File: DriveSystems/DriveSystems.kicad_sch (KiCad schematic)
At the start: 31 parts, among them J1 Raspberry_Pi_4, J2 RJ45, M1 Motor_Servo, M2 Motor_Servo, SW1 SW_Rotary_1x2_MP, U1 RoboClaw Motor Controller, U2 5304 Gear Motor, U3 5VDC 5A UBC-C PSU, U4 24V 5V10A DCDC Stepdown, U5 RoboClaw VClamp, U6 Pwr Res

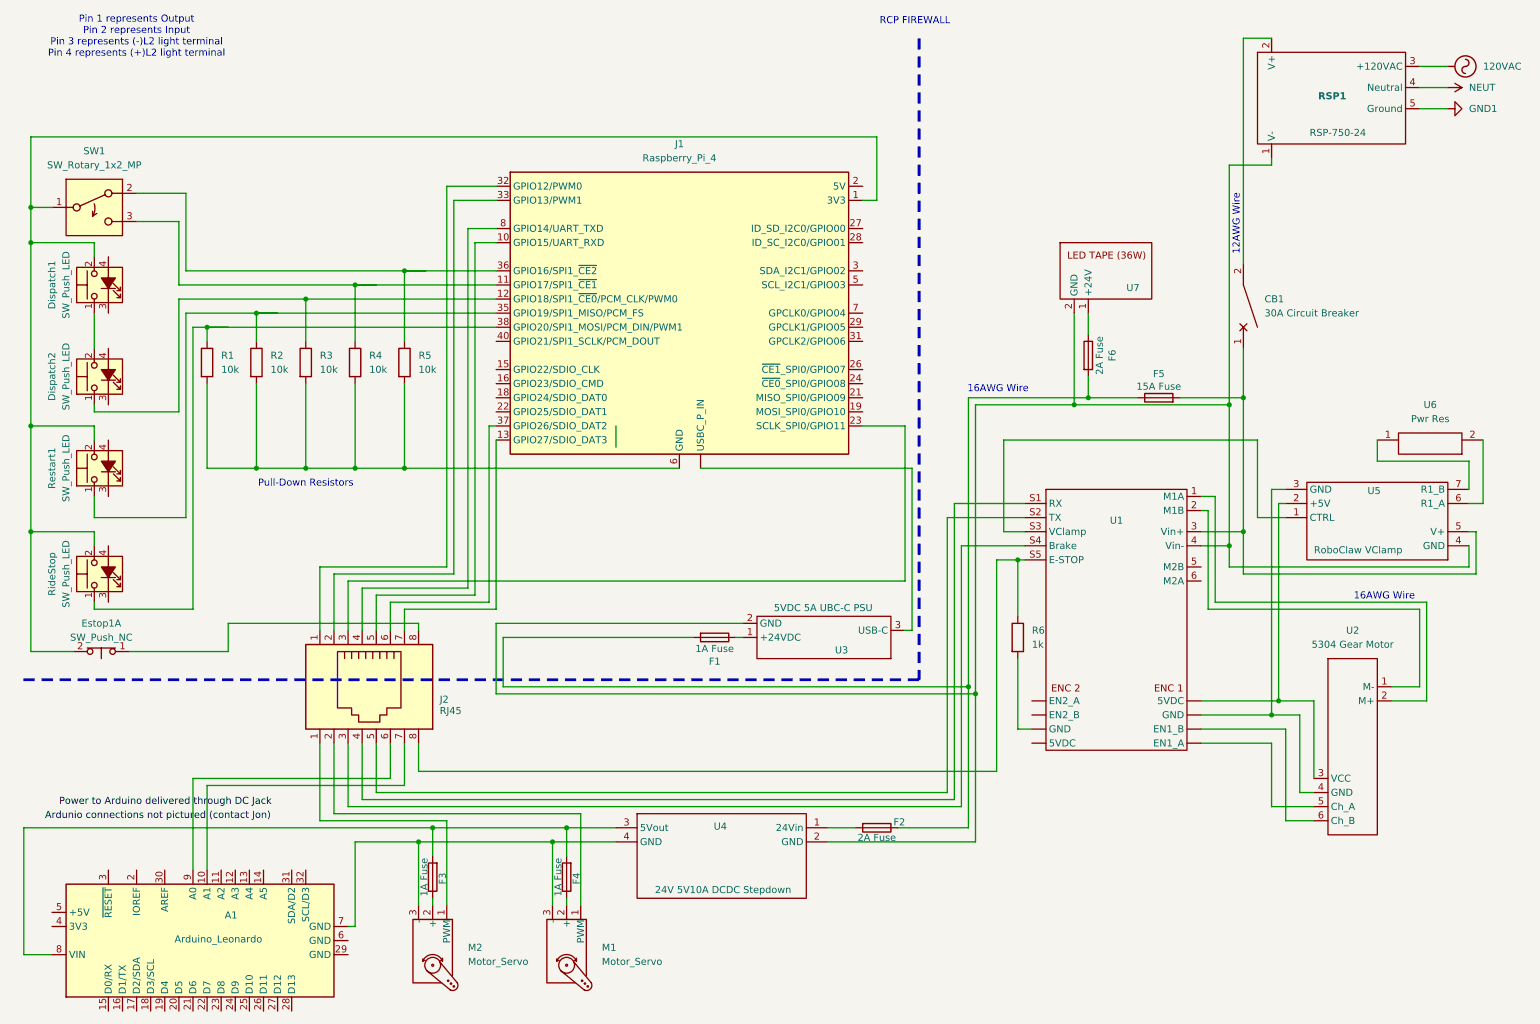
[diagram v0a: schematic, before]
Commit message: Final Cleanup
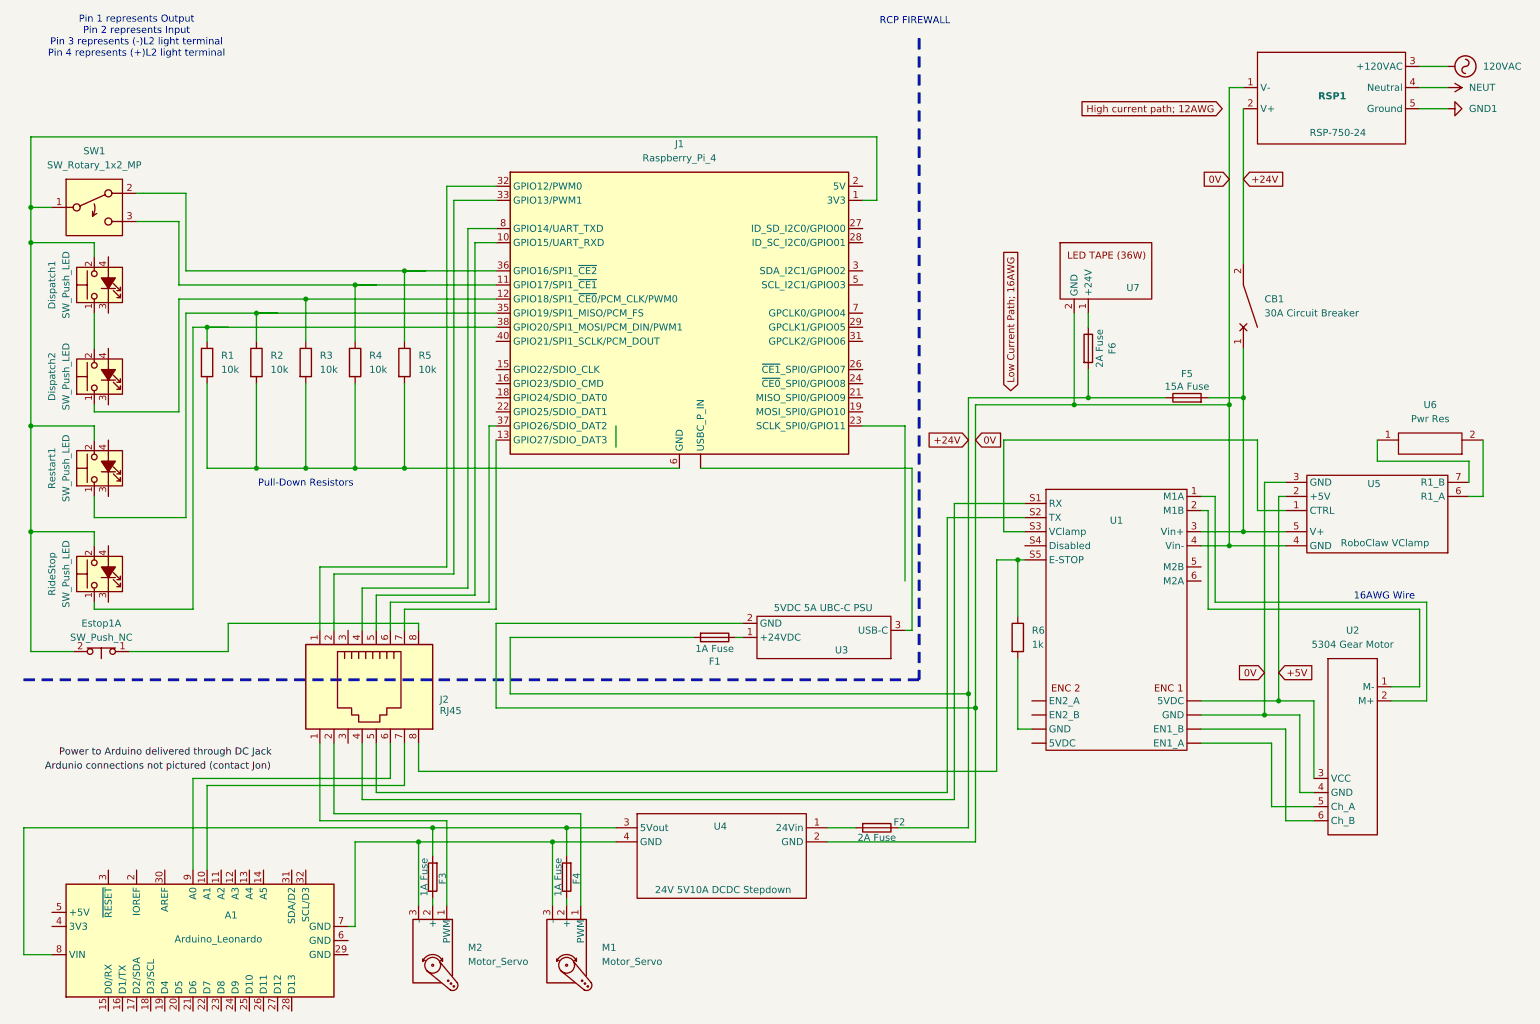
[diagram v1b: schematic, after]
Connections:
- net at J1.23 (SCLK_SPI0/GPIO11): no longer J2.3
- net 0V: now reaches U1. (EN1_A)
- net 0V: now also U1.4 (Vin-), U2.4 (GND), U3.2 (GND), U4.2 (GND), U5.3 (GND), U5.4 (GND), U7.2 (GND)
- net +5V: now reaches U1. (EN1_A), U2.3 (VCC), U5.2 (+5V)
- net at U1.S4 (Disabled): no longer J2.3
- net +24V: now reaches F1.2, F2.1, F5.1, F6.2
- net +24V: now also CB1.2
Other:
- note removed: "12AWG Wire"
- moved on the sheet: F5, F6, U5

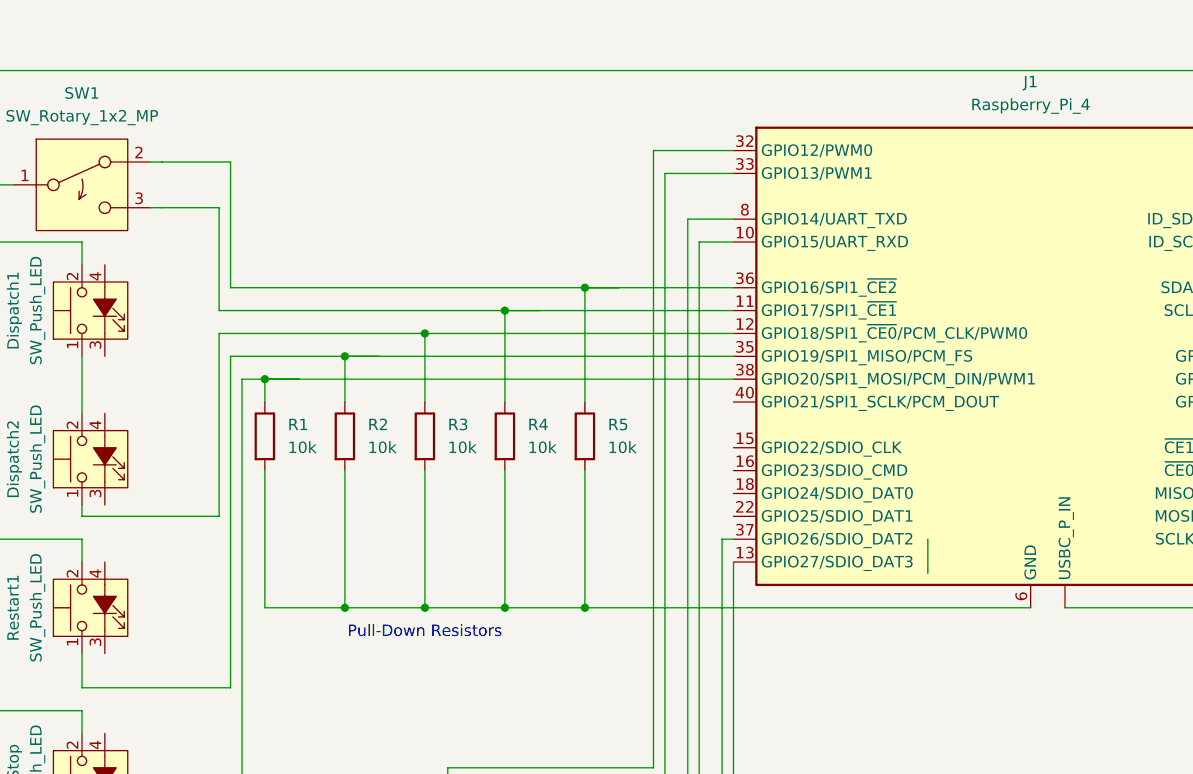
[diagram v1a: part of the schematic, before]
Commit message: NO Switch
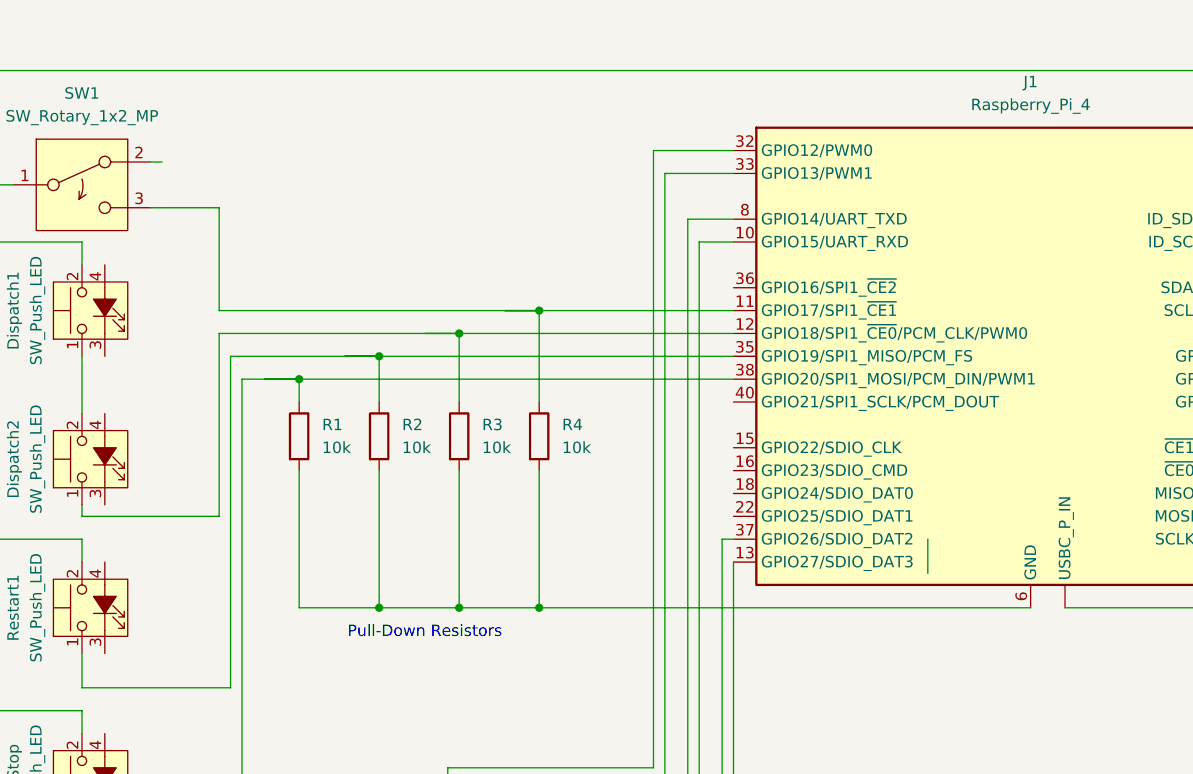
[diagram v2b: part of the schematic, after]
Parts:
- removed R5: 10k, symbol Device:R
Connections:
- net at J1.36 (GPIO16/SPI1_~{CE2}): no longer SW1.2
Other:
- moved on the sheet: R1, R2, R3, R4

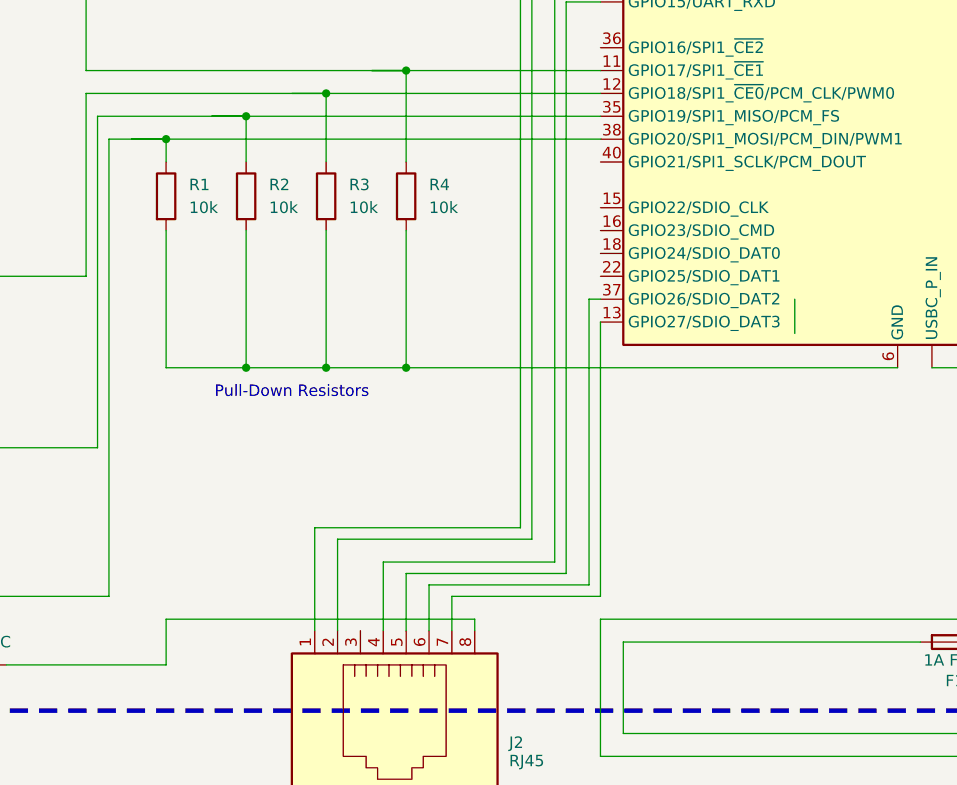
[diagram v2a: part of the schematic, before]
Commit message: Update DriveSystems.kicad_sch
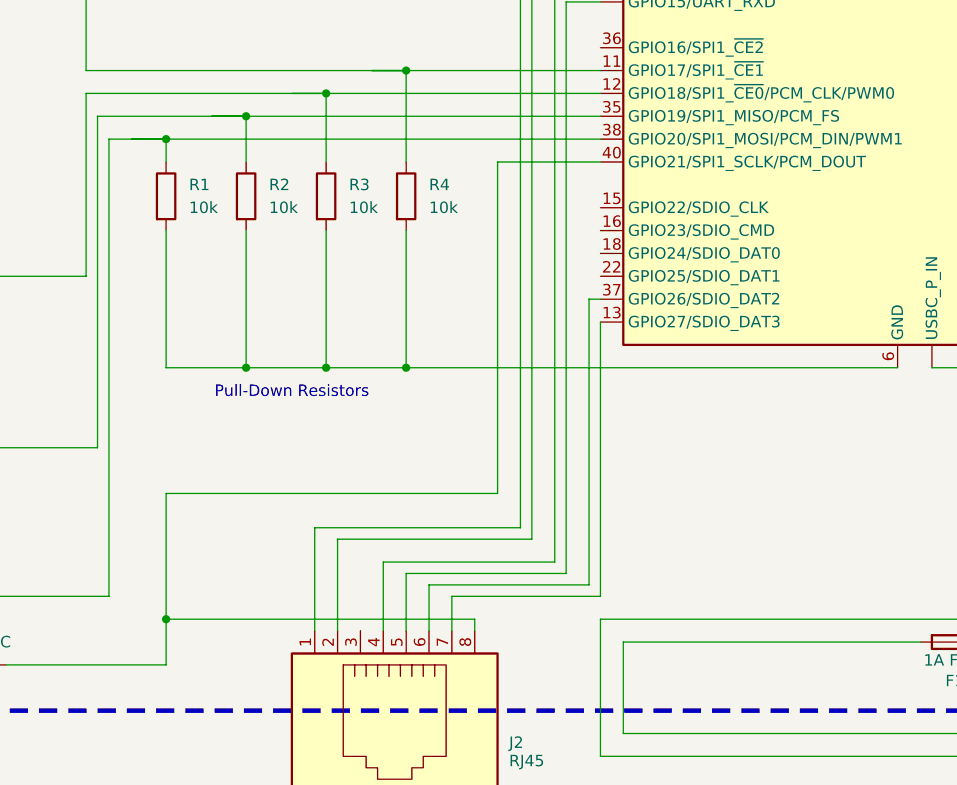
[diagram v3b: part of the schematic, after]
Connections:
- net at J1.40 (GPIO21/SPI1_SCLK/PCM_DOUT): now also Estop1.1, J2.8
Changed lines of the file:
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@@
+	)
+	(junction
+		(at 50.8 125.73)
+		(diameter 0)
+		(color 0 0 0 0)
 	)
 	(junction
@@
 	(wire
 		(pts
+			(xy 50.8 111.76) (xy 87.63 111.76)
+		)
+		(stroke
+			(width 0)
+			(type default)
+			(color 255 0 0 1)
+		)
+	)
+	(wire
+		(pts
 			(xy 59.69 69.85) (xy 99.06 69.85)
 		)
@@
 	(wire
 		(pts
+			(xy 87.63 111.76) (xy 87.63 74.93)
+		)
+		(stroke
+			(width 0)
+			(type default)
+			(color 255 0 0 1)
+		)
+	)
+	(wire
+		(pts
 			(xy 13.97 185.42) (xy 19.05 185.42)
 		)
@@
 		(pts
 			(xy 193.04 114.3) (xy 194.31 114.3)
+		)
+		(stroke
+			(width 0)
+			(type default)
+			(color 255 0 0 1)
+		)
+	)
+	(wire
+		(pts
+			(xy 50.8 125.73) (xy 50.8 111.76)
 		)
 		(stroke
@@
 	(wire
 		(pts
+			(xy 87.63 74.93) (xy 99.06 74.93)
+		)
+		(stroke
+			(width 0)
+			(type default)
+			(color 255 0 0 1)
+		)
+	)
+	(wire
+		(pts
 			(xy 43.18 69.85) (xy 43.18 106.68)
 		)
@@
 		)
 		(stroke
-			(width 0)
-			(type default)
-		)
-	)
-	(wire
-		(pts
-			(xy 120.65 93.98) (xy 120.65 90.17)
-		)
-		(stroke
